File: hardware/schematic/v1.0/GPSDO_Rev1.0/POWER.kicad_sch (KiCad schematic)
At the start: 28 parts, among them CN1 LAIL-PHC2_54-2P-01-XH-L, U14 TPS7A5201RPSR, U16 TPS7A5201RPSR

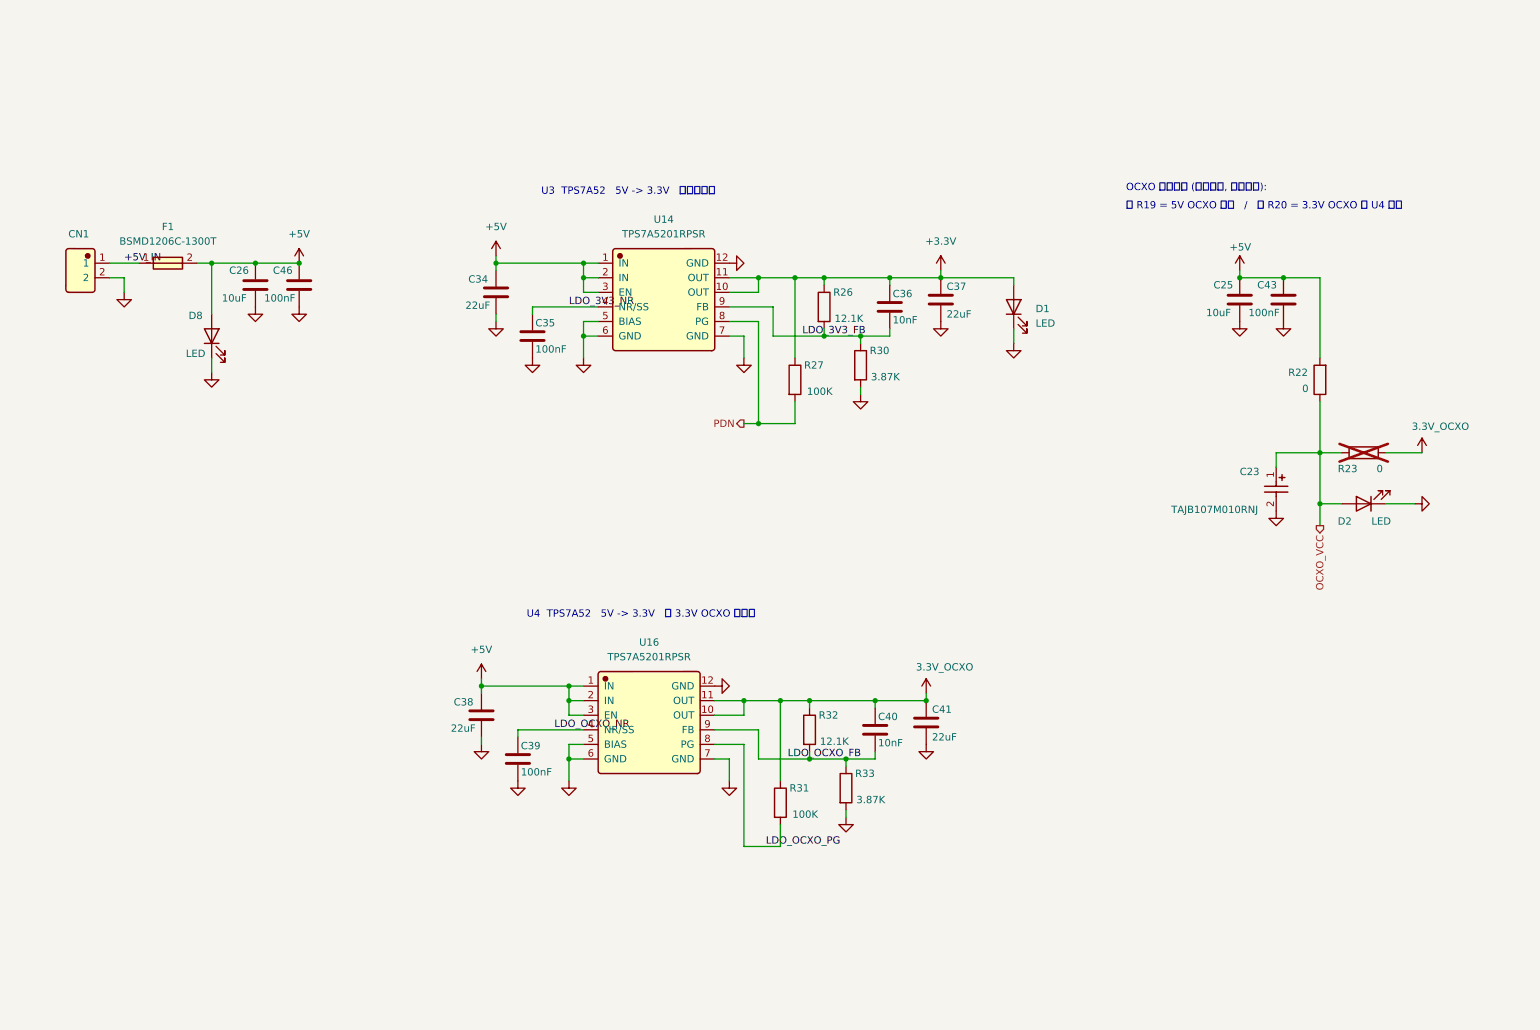
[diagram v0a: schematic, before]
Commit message: sch update
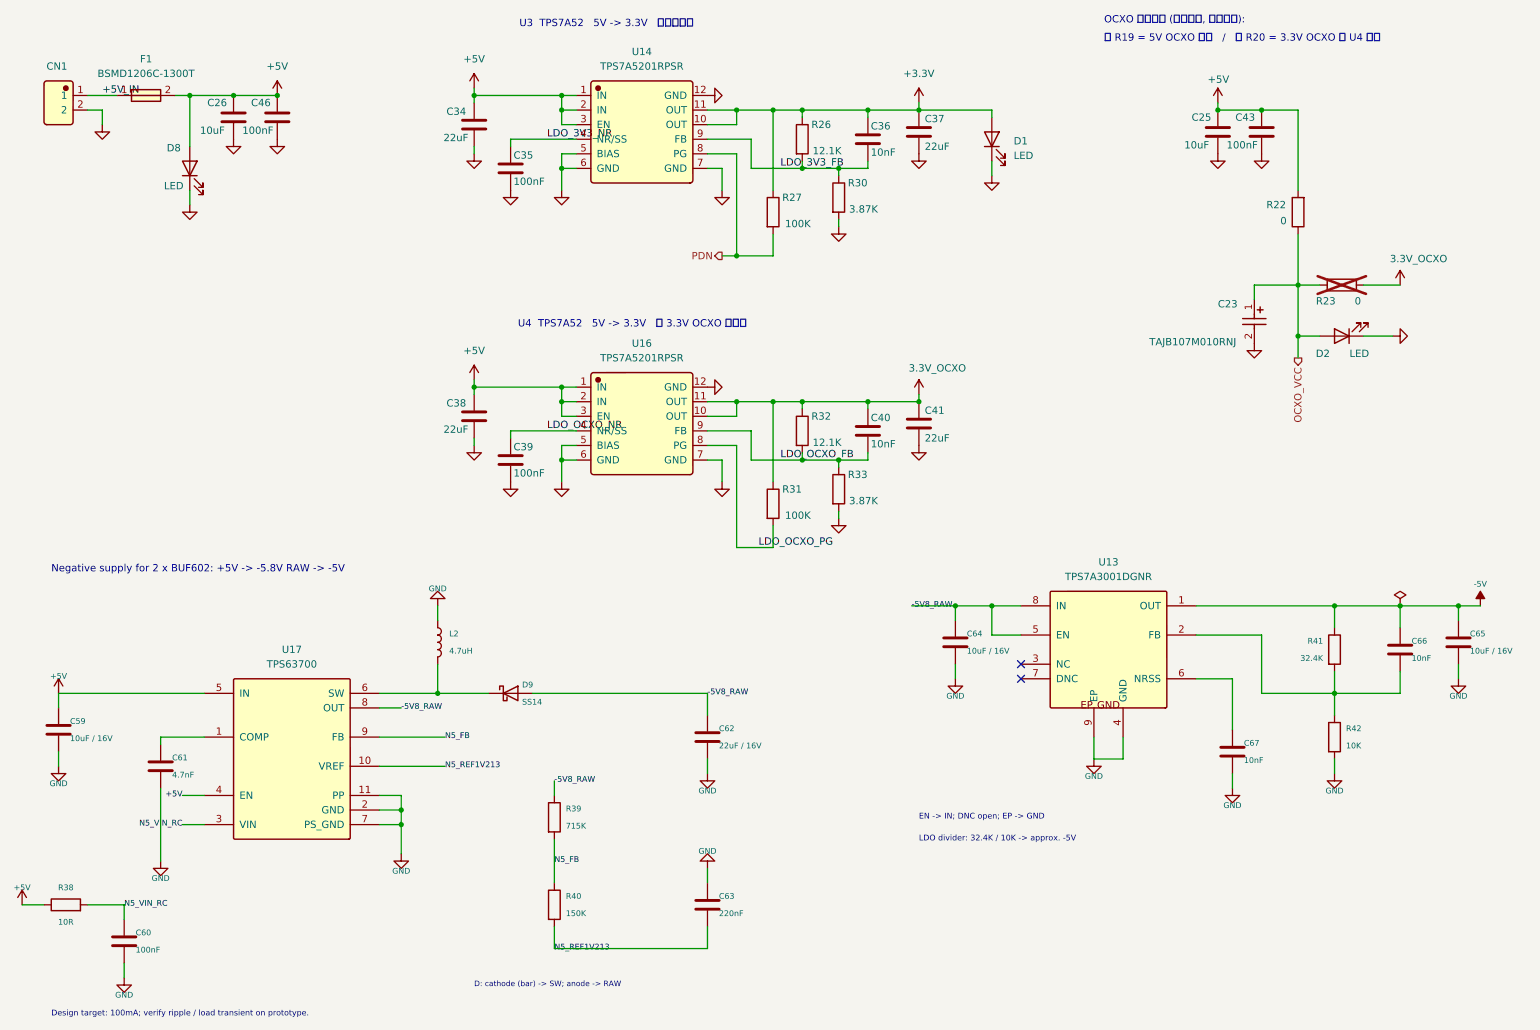
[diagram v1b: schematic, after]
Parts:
- added C59, C64, C65: 10uF / 16V, Capacitor_SMD:C_0805_2012Metric, symbol GPSDO_Rev1.0:C
- added C60: 100nF, Capacitor_SMD:C_0603_1608Metric, symbol GPSDO_Rev1.0:C
- added C61: 4.7nF, Capacitor_SMD:C_0603_1608Metric, symbol GPSDO_Rev1.0:C
- added C62: 22uF / 16V, Capacitor_SMD:C_1210_3225Metric, symbol GPSDO_Rev1.0:C
- added C63: 220nF, Capacitor_SMD:C_0603_1608Metric, symbol GPSDO_Rev1.0:C
- added C66, C67: 10nF, Capacitor_SMD:C_0603_1608Metric, symbol GPSDO_Rev1.0:C
- added D9: SS14, Diode_SMD:D_SMA, symbol GPSDO_Rev1.0:D_Schottky
- added L2: 4.7uH, Inductor_SMD:L_Coilcraft_LPS4018, symbol GPSDO_Rev1.0:L
- added R38: 10R, Resistor_SMD:R_0603_1608Metric, symbol GPSDO_Rev1.0:R
- added R39: 715K, Resistor_SMD:R_0603_1608Metric, symbol GPSDO_Rev1.0:R
- added R40: 150K, Resistor_SMD:R_0603_1608Metric, symbol GPSDO_Rev1.0:R
- added R41: 32.4K, Resistor_SMD:R_0603_1608Metric, symbol GPSDO_Rev1.0:R
- added R42: 10K, Resistor_SMD:R_0603_1608Metric, symbol GPSDO_Rev1.0:R
- added U13: TPS7A3001DGNR, GPSDO_Rev1.0:TPS7A3001DGNR, symbol GPSDO_Rev1.0:TPS7A3001DGNR
- added U17: TPS63700, GPSDO_Rev1.0:TPS63700, symbol GPSDO_Rev1.0:TPS63700
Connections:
- net +5V: now also C59.1, R38.1, U17.4 (EN), U17.5 (IN)
- net GND: now also C59.2, C60.2, C61.2, C62.2, C63.1, C64.2, C65.2, C67.2, L2.1, R42.2, U13.4 (GND), U13.9 (EP), U17.11 (PP), U17.2 (GND), U17.7 (PS_GND)
- new net: D9.1 (K), L2.2, U17.6 (SW)
- new net: C61.1, U17.1 (COMP)
- new net: C66.2, R41.2, R42.1, U13.2 (FB)
- new net: C67.1, U13.6 (NRSS)
- new net -5V: C65.1, C66.1, R41.1, U13.1 (OUT)
- new net -5V8_RAW: C62.1, C64.1, D9.2 (A), R39.1, U13.5 (EN), U13.8 (IN), U17.8 (OUT)
- new net N5_FB: R39.2, R40.1, U17.9 (FB)
- new net N5_REF1V213: C63.2, R40.2, U17.10 (VREF)
- new net N5_VIN_RC: C60.1, R38.2, U17.3 (VIN)
- no-connect marks 0 -> 2
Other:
- note added: "D: cathode (bar) -> SW; anode -> RAW"
- note added: "Design target: 100mA; verify ripple / load transient on prototype."
- note added: "EN -> IN; DNC open; EP -> GND"
- note added: "LDO divider: 32.4K / 10K -> approx. -5V"
- note added: "Negative supply for 2 x BUF602: +5V -> -5.8V RAW -> -5V"
- moved on the sheet: C23, C25, C26, C34, C35, C36, C37, C38, C39, C40, C41, C43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

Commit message: sch update
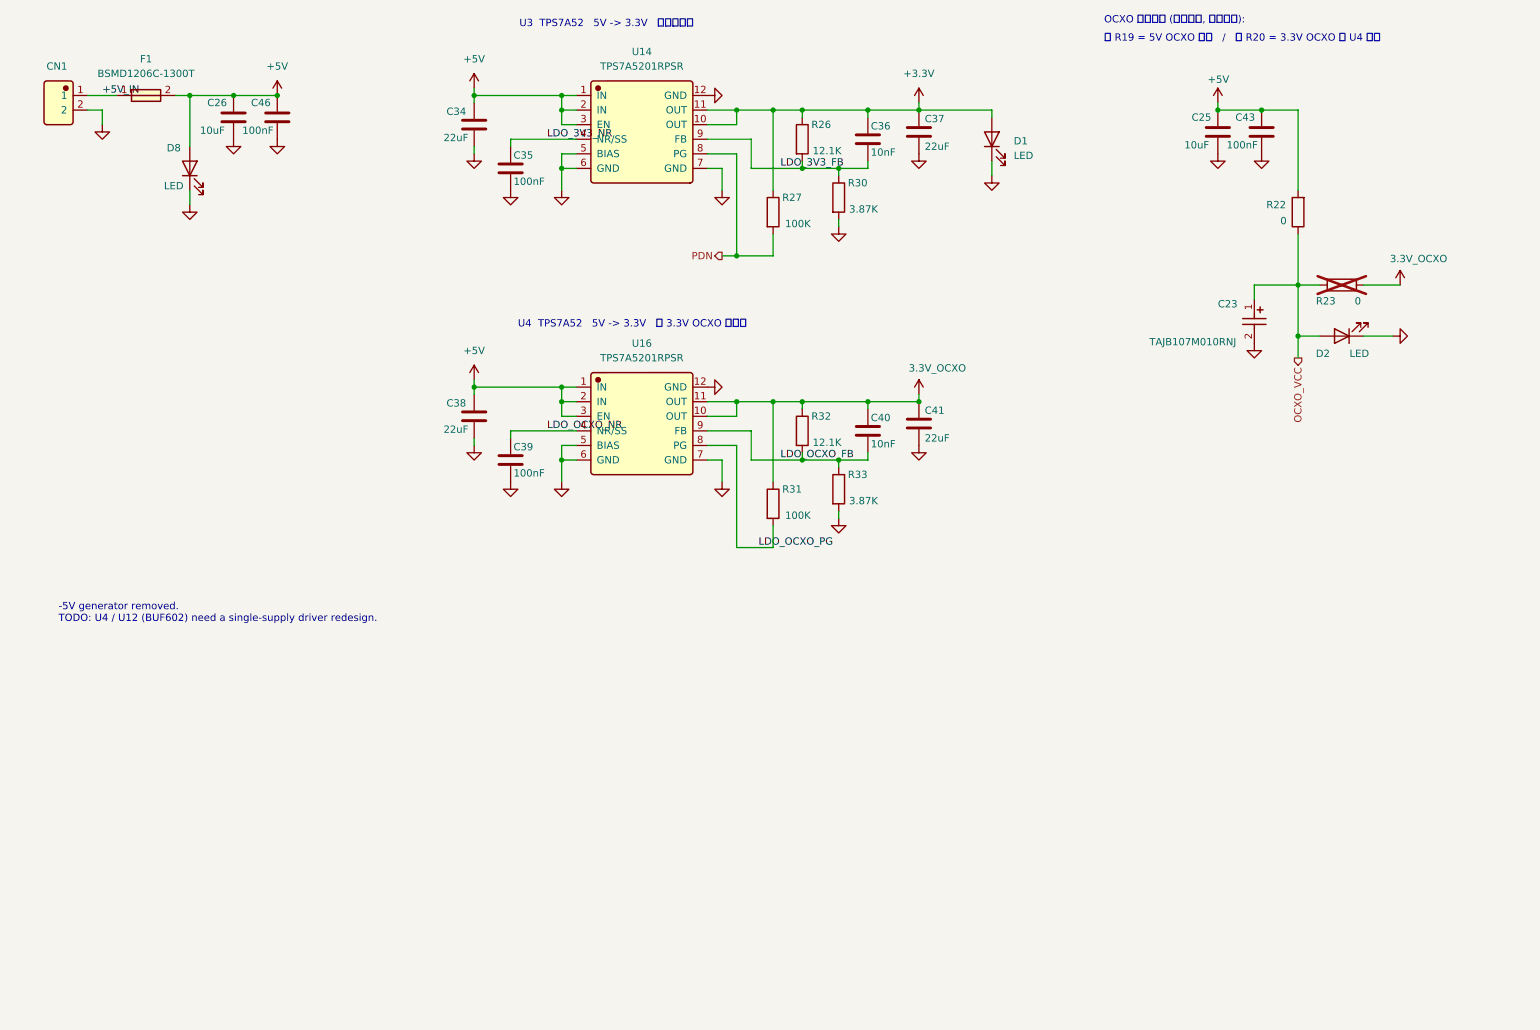
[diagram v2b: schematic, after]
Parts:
- removed C59, C64, C65: 10uF / 16V, Capacitor_SMD:C_0805_2012Metric, symbol GPSDO_Rev1.0:C
- removed C60: 100nF, Capacitor_SMD:C_0603_1608Metric, symbol GPSDO_Rev1.0:C
- removed C61: 4.7nF, Capacitor_SMD:C_0603_1608Metric, symbol GPSDO_Rev1.0:C
- removed C62: 22uF / 16V, Capacitor_SMD:C_1210_3225Metric, symbol GPSDO_Rev1.0:C
- removed C63: 220nF, Capacitor_SMD:C_0603_1608Metric, symbol GPSDO_Rev1.0:C
- removed C66, C67: 10nF, Capacitor_SMD:C_0603_1608Metric, symbol GPSDO_Rev1.0:C
- removed D9: SS14, Diode_SMD:D_SMA, symbol GPSDO_Rev1.0:D_Schottky
- removed L2: 4.7uH, Inductor_SMD:L_Coilcraft_LPS4018, symbol GPSDO_Rev1.0:L
- removed R38: 10R, Resistor_SMD:R_0603_1608Metric, symbol GPSDO_Rev1.0:R
- removed R39: 715K, Resistor_SMD:R_0603_1608Metric, symbol GPSDO_Rev1.0:R
- removed R40: 150K, Resistor_SMD:R_0603_1608Metric, symbol GPSDO_Rev1.0:R
- removed R41: 32.4K, Resistor_SMD:R_0603_1608Metric, symbol GPSDO_Rev1.0:R
- removed R42: 10K, Resistor_SMD:R_0603_1608Metric, symbol GPSDO_Rev1.0:R
- removed U13: TPS7A3001DGNR, GPSDO_Rev1.0:TPS7A3001DGNR, symbol GPSDO_Rev1.0:TPS7A3001DGNR
- removed U17: TPS63700, GPSDO_Rev1.0:TPS63700, symbol GPSDO_Rev1.0:TPS63700
- C23: footprint JLCImport:TAJB107M010RNJ -> GPSDO_Rev1.0:TAJB107M010RNJ; symbol JLCImport:TAJB107M010RNJ -> GPSDO_Rev1.0:TAJB107M010RNJ
- C34, C37, C38, C41: symbol GPSDO_Rev1.0:C -> GPSDO_Rev1.0:C__C_0805_2012Metric
- C35, C36, C39, C40, C43, C46: symbol GPSDO_Rev1.0:C -> GPSDO_Rev1.0:C__C_0402_1005Metric
- F1: footprint JLCImport:BSMD1206C-1300T -> GPSDO_Rev1.0:BSMD1206C-1300T; symbol JLCImport:BSMD1206C-1300T -> GPSDO_Rev1.0:BSMD1206C-1300T
- R22, R23: symbol GPSDO_Rev1.0:R -> GPSDO_Rev1.0:R__R_0805_2012Metric
- R26, R27, R30, R31, R32, R33: symbol GPSDO_Rev1.0:R -> GPSDO_Rev1.0:R__R_0402_1005Metric
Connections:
- no-connect marks 2 -> 0
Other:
- note added: "-5V generator removed. TODO: U4 / U12 (BUF602) need a single-supply driver redesign."
- note removed: "D: cathode (bar) -> SW; anode -> RAW"
- note removed: "Design target: 100mA; verify ripple / load transient on prototype."
- note removed: "EN -> IN; DNC open; EP -> GND"
- note removed: "LDO divider: 32.4K / 10K -> approx. -5V"
- note removed: "Negative supply for 2 x BUF602: +5V -> -5.8V RAW -> -5V"
